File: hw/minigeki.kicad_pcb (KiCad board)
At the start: 2 copper layers, 52 x 56.1 mm, 29 parts, among them J1 USB_C_Receptacle_USB2.0, J2 Conn_01x02, U1 NCP1117-3.3_SOT223, U2 W25Q128JVS, U3 RP2040, Y1 ABLS-12.000MHZ-B4-T

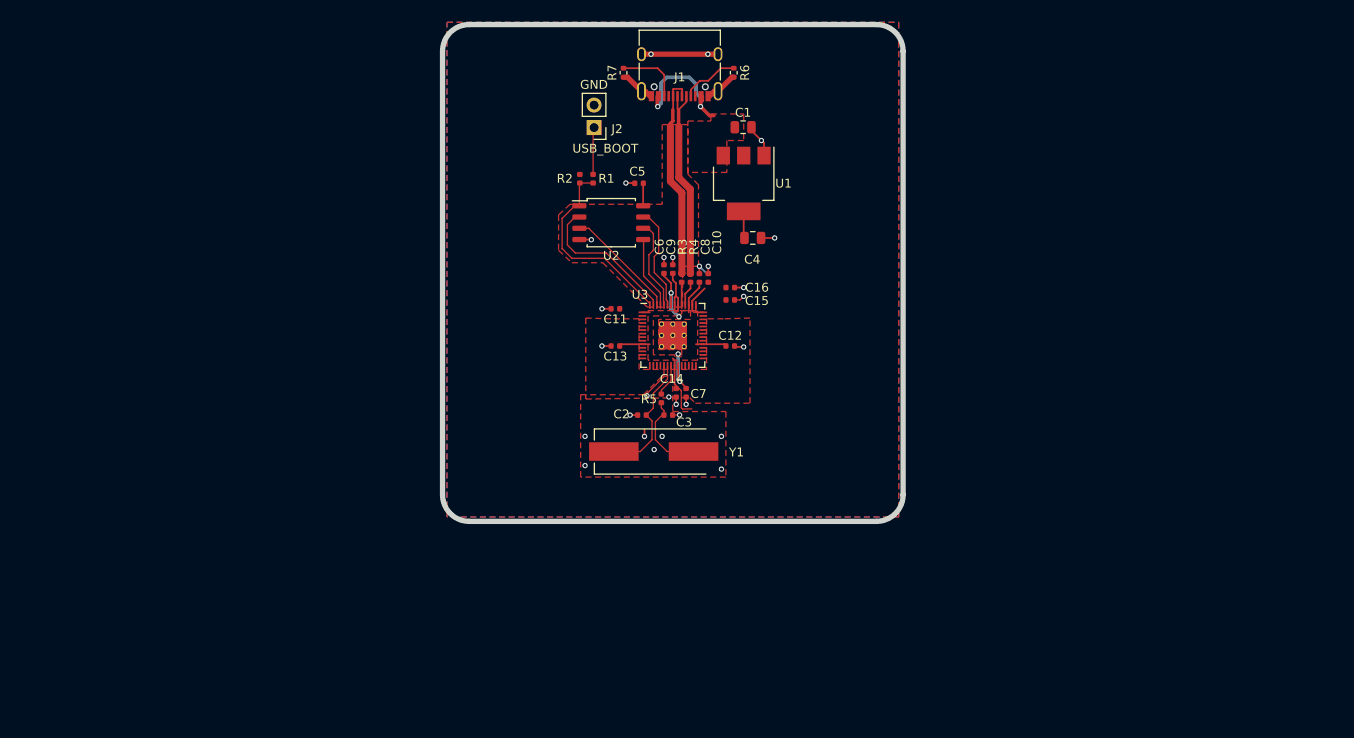
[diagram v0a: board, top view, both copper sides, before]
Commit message: hw: finish main routing
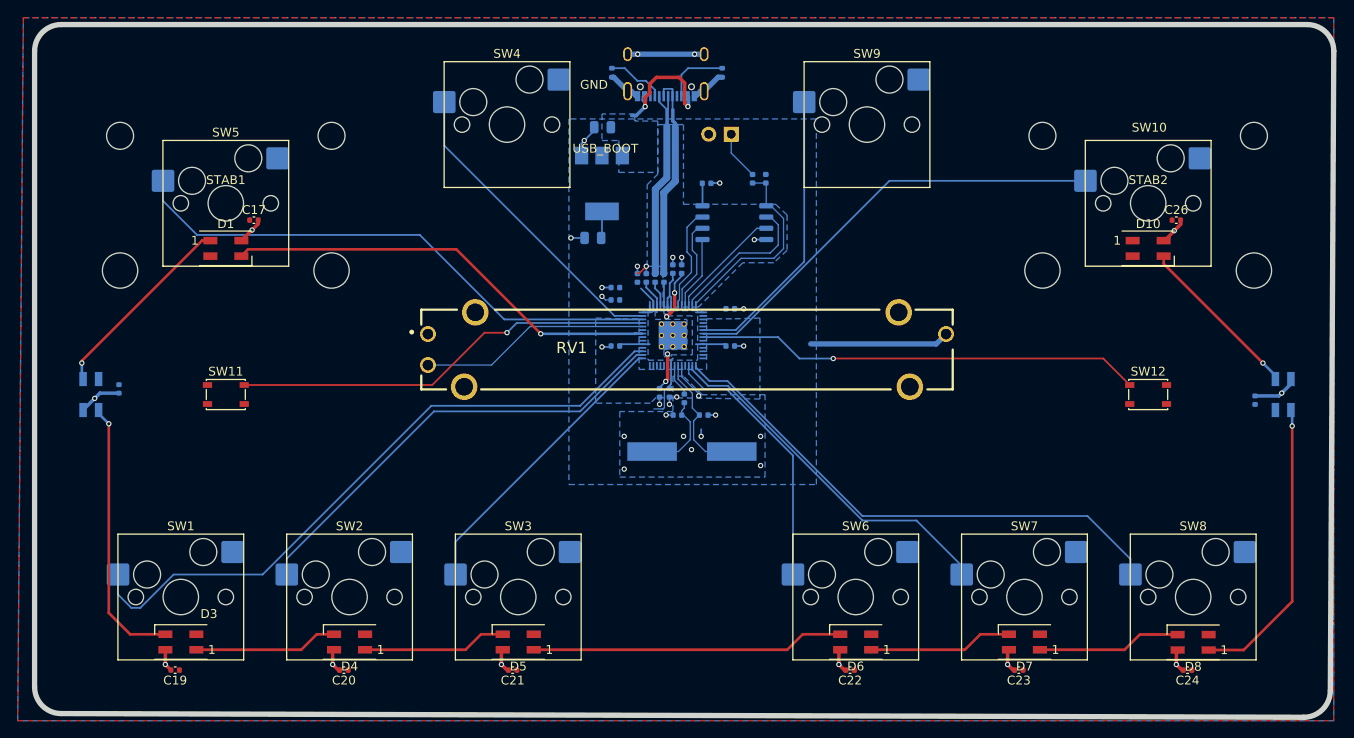
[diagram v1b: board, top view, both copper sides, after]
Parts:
- added C17: 100n, Capacitor_SMD:C_0402_1005Metric, F.Cu at (52.7, 87.0)
- added C18: 100n, Capacitor_SMD:C_0402_1005Metric, B.Cu at (37.5, 106.0)
- added C19: 100n, Capacitor_SMD:C_0402_1005Metric, F.Cu at (43.8, 137.8)
- added C20: 100n, Capacitor_SMD:C_0402_1005Metric, F.Cu at (62.9, 137.8)
- added C21: 100n, Capacitor_SMD:C_0402_1005Metric, F.Cu at (81.9, 137.8)
- added C22: 100n, Capacitor_SMD:C_0402_1005Metric, F.Cu at (120.0, 137.8)
- added C23: 100n, Capacitor_SMD:C_0402_1005Metric, F.Cu at (139.1, 137.8)
- added C24: 100n, Capacitor_SMD:C_0402_1005Metric, F.Cu at (158.1, 137.8)
- added C25: 100n, Capacitor_SMD:C_0402_1005Metric, B.Cu at (165.7, 107.3)
- added C26: 100n, Capacitor_SMD:C_0402_1005Metric, F.Cu at (156.8, 87.0)
- added D1: SK6812MINI, LED_SMD:LED_SK6812MINI_PLCC4_3.5x3.5mm_P1.75mm, F.Cu at (49.5, 90.2)
- added D10: SK6812MINI, LED_SMD:LED_SK6812MINI_PLCC4_3.5x3.5mm_P1.75mm, F.Cu at (153.7, 90.2)
- added D2: SK6812MINI, LED_SMD:LED_SK6812MINI_PLCC4_3.5x3.5mm_P1.75mm, B.Cu at (34.3, 106.7)
- added D3: SK6812MINI, LED_SMD:LED_SK6812MINI_PLCC4_3.5x3.5mm_P1.75mm, F.Cu at (44.5, 134.6)
- added D4: SK6812MINI, LED_SMD:LED_SK6812MINI_PLCC4_3.5x3.5mm_P1.75mm, F.Cu at (63.5, 134.6)
- added D5: SK6812MINI, LED_SMD:LED_SK6812MINI_PLCC4_3.5x3.5mm_P1.75mm, F.Cu at (82.5, 134.6)
- added D6: SK6812MINI, LED_SMD:LED_SK6812MINI_PLCC4_3.5x3.5mm_P1.75mm, F.Cu at (120.7, 134.6)
- added D7: SK6812MINI, LED_SMD:LED_SK6812MINI_PLCC4_3.5x3.5mm_P1.75mm, F.Cu at (139.7, 134.6)
- added D8: SK6812MINI, LED_SMD:LED_SK6812MINI_PLCC4_3.5x3.5mm_P1.75mm, F.Cu at (158.8, 134.7)
- added D9: SK6812MINI, LED_SMD:LED_SK6812MINI_PLCC4_3.5x3.5mm_P1.75mm, B.Cu at (168.9, 106.7)
- added RV1: PTA4543-2015DPB103, PTAXX33:PTAXX43, F.Cu at (101.6, 101.6)
- added STAB1: Stabilizer_Cherry_MX_2.00u, Mounting_Keyboard_Stabilizer:Stabilizer_Cherry_MX_2.00u, F.Cu at (49.5, 84.5)
- added STAB2: Stabilizer_Cherry_MX_2.00u, Mounting_Keyboard_Stabilizer:Stabilizer_Cherry_MX_2.00u, F.Cu at (153.7, 84.5)
- added SW1: LEFT_R, Switch_Keyboard_Hotswap_Kailh:SW_Hotswap_Kailh_MX_1.00u, F.Cu at (44.5, 129.5)
- added SW10: RIGHT_WALL, Switch_Keyboard_Hotswap_Kailh:SW_Hotswap_Kailh_MX_2.00u, F.Cu at (153.7, 85.1)
- added SW11: MACRO_1, Button_Switch_SMD:SW_SPST_PTS810, F.Cu at (49.5, 106.7)
- added SW12: MACRO_2, Button_Switch_SMD:SW_SPST_PTS810, F.Cu at (153.7, 106.7)
- added SW2: LEFT_G, Switch_Keyboard_Hotswap_Kailh:SW_Hotswap_Kailh_MX_1.00u, F.Cu at (63.5, 129.5)
- added SW3: LEFT_B, Switch_Keyboard_Hotswap_Kailh:SW_Hotswap_Kailh_MX_1.00u, F.Cu at (82.5, 129.5)
- added SW4: LEFT_START, Switch_Keyboard_Hotswap_Kailh:SW_Hotswap_Kailh_MX_1.00u, F.Cu at (81.3, 76.2)
- added SW5: LEFT_WALL, Switch_Keyboard_Hotswap_Kailh:SW_Hotswap_Kailh_MX_2.00u, F.Cu at (49.5, 85.1)
- added SW6: RIGHT_R, Switch_Keyboard_Hotswap_Kailh:SW_Hotswap_Kailh_MX_1.00u, F.Cu at (120.7, 129.5)
- added SW7: RIGHT_G, Switch_Keyboard_Hotswap_Kailh:SW_Hotswap_Kailh_MX_1.00u, F.Cu at (139.7, 129.5)
- added SW8: RIGHT_B, Switch_Keyboard_Hotswap_Kailh:SW_Hotswap_Kailh_MX_1.00u, F.Cu at (158.8, 129.5)
- added SW9: RIGHT_START, Switch_Keyboard_Hotswap_Kailh:SW_Hotswap_Kailh_MX_1.00u, F.Cu at (121.9, 76.2)
- C1, C10, C11, C12, C13, C14, C15, C16, C2, C3, C4, C5, C6, C7, C8, C9, J1, J2, R1, R2, R3, R4, R5, R6, R7, U1, U2, U3, Y1: moved to B.Cu
- moved R2 21.0 mm to (110.5, 82.3)
- moved C4 18.1 mm to (91.0, 89.0), turned to 180 degrees
- moved R1 18.0 mm to (109.0, 82.3)
- moved U1 16.0 mm to (92.0, 82.8)
- moved C1 15.9 mm to (92.1, 76.5), turned to 180 degrees
- moved J2 15.5 mm to (106.6, 77.3), turned to 90 degrees
- moved U2 13.9 mm to (107.0, 87.3), turned to 180 degrees
- moved R6 13.8 mm to (93.1, 70.3)
- moved C11 13.0 mm to (106.5, 97.0), turned to 0 degrees
- moved C12 13.0 mm to (93.5, 101.2), turned to 180 degrees
- moved C13 13.0 mm to (106.5, 101.2), turned to 0 degrees
- moved C15 13.0 mm to (93.5, 96.0), turned to 180 degrees
- moved C16 13.0 mm to (93.5, 94.6), turned to 180 degrees
- moved R7 11.1 mm to (105.6, 70.3)
- moved C10 8.00 mm to (96.0, 93.5)
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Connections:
- U3 pad 11: /GPIO8 -> unconnected-(U3-Pad11)
- U3 pad 12: /GPIO9 -> unconnected-(U3-Pad12)
- U3 pad 13: /GPIO10 -> unconnected-(U3-Pad13)
- U3 pad 14: /GPIO11 -> unconnected-(U3-Pad14)
- U3 pad 15: /GPIO12 -> /RIGHT_B
- U3 pad 16: /GPIO13 -> /RIGHT_G
- U3 pad 17: /GPIO14 -> /RIGHT_R
- U3 pad 18: /GPIO15 -> unconnected-(U3-Pad18)
- U3 pad 2: /GPIO0 -> unconnected-(U3-Pad2)
- U3 pad 27: /GPIO16 -> unconnected-(U3-Pad27)
- U3 pad 28: /GPIO17 -> unconnected-(U3-Pad28)
- U3 pad 29: /GPIO18 -> /LEFT_B
- U3 pad 3: /GPIO1 -> unconnected-(U3-Pad3)
- U3 pad 30: /GPIO19 -> /LEFT_G
- U3 pad 31: /GPIO20 -> /LEFT_R
- U3 pad 32: /GPIO21 -> unconnected-(U3-Pad32)
- U3 pad 34: /GPIO22 -> unconnected-(U3-Pad34)
- U3 pad 35: /GPIO23 -> unconnected-(U3-Pad35)
- U3 pad 36: /GPIO24 -> /LED_DIN
- U3 pad 37: /GPIO25 -> unconnected-(U3-Pad37)
- U3 pad 39: /GPIO27_ADC1 -> /MACRO_1
- U3 pad 4: /GPIO2 -> unconnected-(U3-Pad4)
- U3 pad 40: /GPIO28_ADC2 -> /LEFT_WALL
- U3 pad 41: /GPIO29_ADC3 -> /LEFT_START
- U3 pad 5: /GPIO3 -> unconnected-(U3-Pad5)
- U3 pad 6: /GPIO4 -> /RIGHT_START
- U3 pad 7: /GPIO5 -> /RIGHT_WALL
- U3 pad 8: /GPIO6 -> /MACRO2
- U3 pad 9: /GPIO7 -> unconnected-(U3-Pad9)
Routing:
- net /LEFT_R: track 0.00 -> 74.1 mm
- net /LEFT_WALL: track 0.00 -> 61.9 mm
- net /RIGHT_B: track 0.00 -> 60.0 mm
- net /LEFT_G: track 0.00 -> 51.5 mm
- net /MACRO2: track 0.00 -> 50.4 mm, vias 0 -> 1
- net /RIGHT_WALL: track 0.00 -> 50.3 mm
- net /LED_DIN: track 0.00 -> 49.6 mm, vias 0 -> 1
- net /MACRO_1: track 0.00 -> 47.9 mm, vias 0 -> 1
- net /RIGHT_G: track 0.00 -> 41.0 mm
- net Net-(D5-Pad1): track 0.00 -> 35.3 mm
- net /LEFT_START: track 0.00 -> 35.2 mm
- net /LEFT_B: track 0.00 -> 33.4 mm
- net Net-(D8-Pad1): track 0.00 -> 33.4 mm, vias 0 -> 1
- net /RIGHT_START: track 0.00 -> 32.6 mm
- net Net-(D2-Pad1): track 0.00 -> 30.8 mm, vias 0 -> 1
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- added copper zone on B.Cu, net +1V1
- added copper zone on B.Cu, net +3V3
- added copper zone on B.Cu, net VBUS
- removed copper zone on F.Cu, net +1V1
- removed copper zone on F.Cu, net +3V3
- removed copper zone on F.Cu, net VBUS
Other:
- board size 52 x 56.1 mm -> 146.7 x 78.2 mm
